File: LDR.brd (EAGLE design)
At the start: 39.8 x 21.5 mm, 13 parts, among them J1 CONECTOR_MACHO, J2 CONECTOR_FEMEA, U1 TL494BD

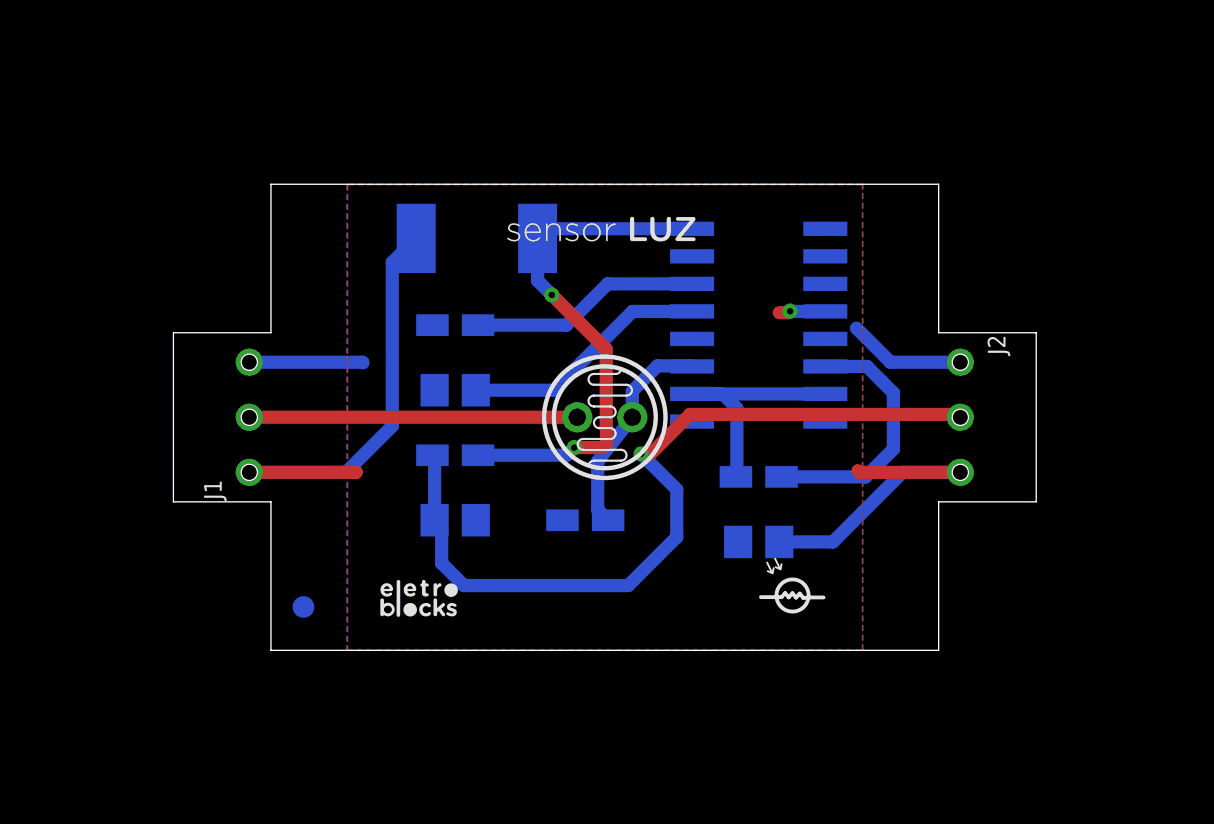
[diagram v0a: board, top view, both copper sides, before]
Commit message: V1.1.1
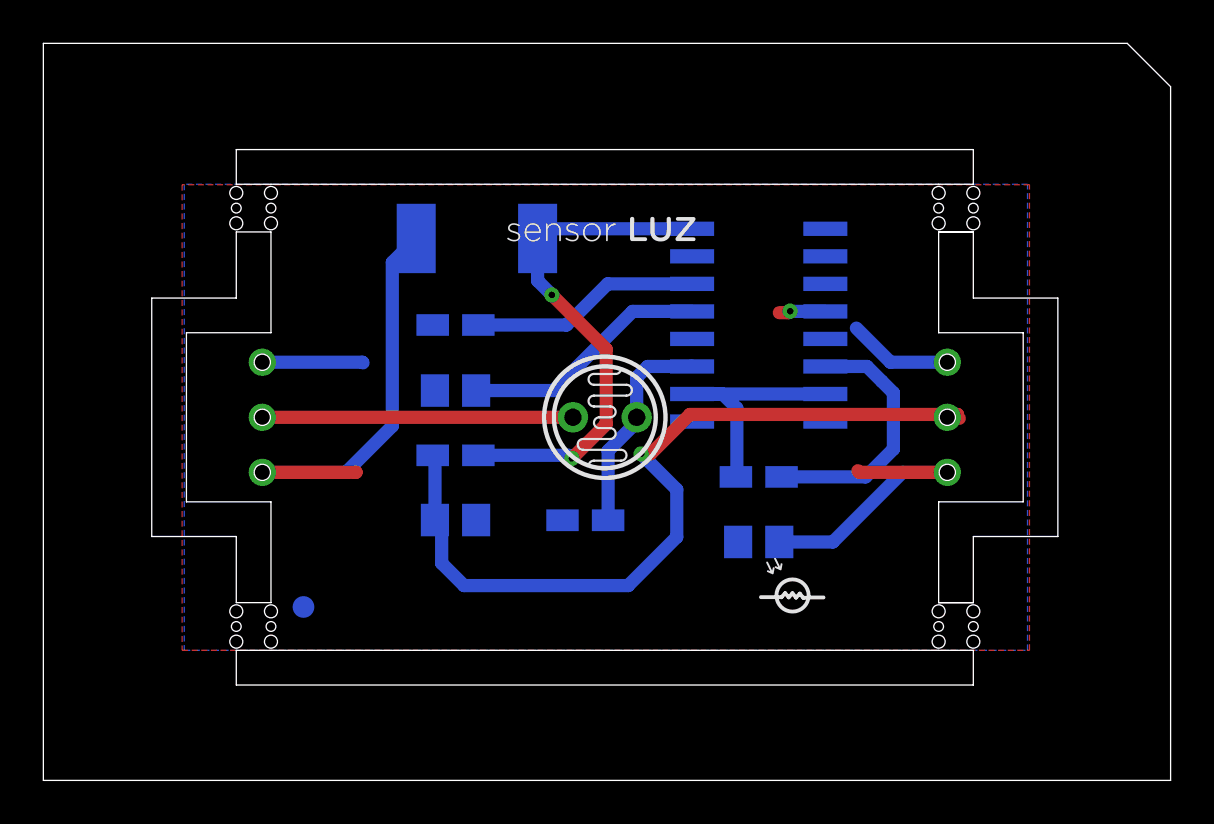
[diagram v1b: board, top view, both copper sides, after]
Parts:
- added U$2, U$3, U$4, U$5: (no value), Eletroblocks Lib:STAMP_DUPLO
- J1: device Eletroblocks Lib:3CONECTOR -> Eletroblocks Lib:MALE
- J2: device Eletroblocks Lib:3CONECTOR -> Eletroblocks Lib:FEMALE
- moved J2 0.60 mm to (27.7, 10.8)
- moved J1 0.60 mm to (-3.90, 10.8)
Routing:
- net VCC: track 38.1 -> 35.7 mm
- net GND: track 10.7 -> 9.50 mm
- net SIGNAL_IN: track 15.1 -> 14.3 mm
- net SIGNAL_OUT: track 37.5 -> 38.3 mm
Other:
- board size 39.8 x 21.5 mm -> 52 x 34 mm
- board text added: "V1.1.1"
- board text removed: "V1.1.0"
